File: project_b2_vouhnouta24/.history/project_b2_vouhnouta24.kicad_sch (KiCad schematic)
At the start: 13 parts, among them J1 AVR-ISP-10, J2 Micro_SD_Card, U1 ATmega328-P-A, U2 ADP2108AUJ-3.3, U3 TXB0104D, Y1 16Mhz

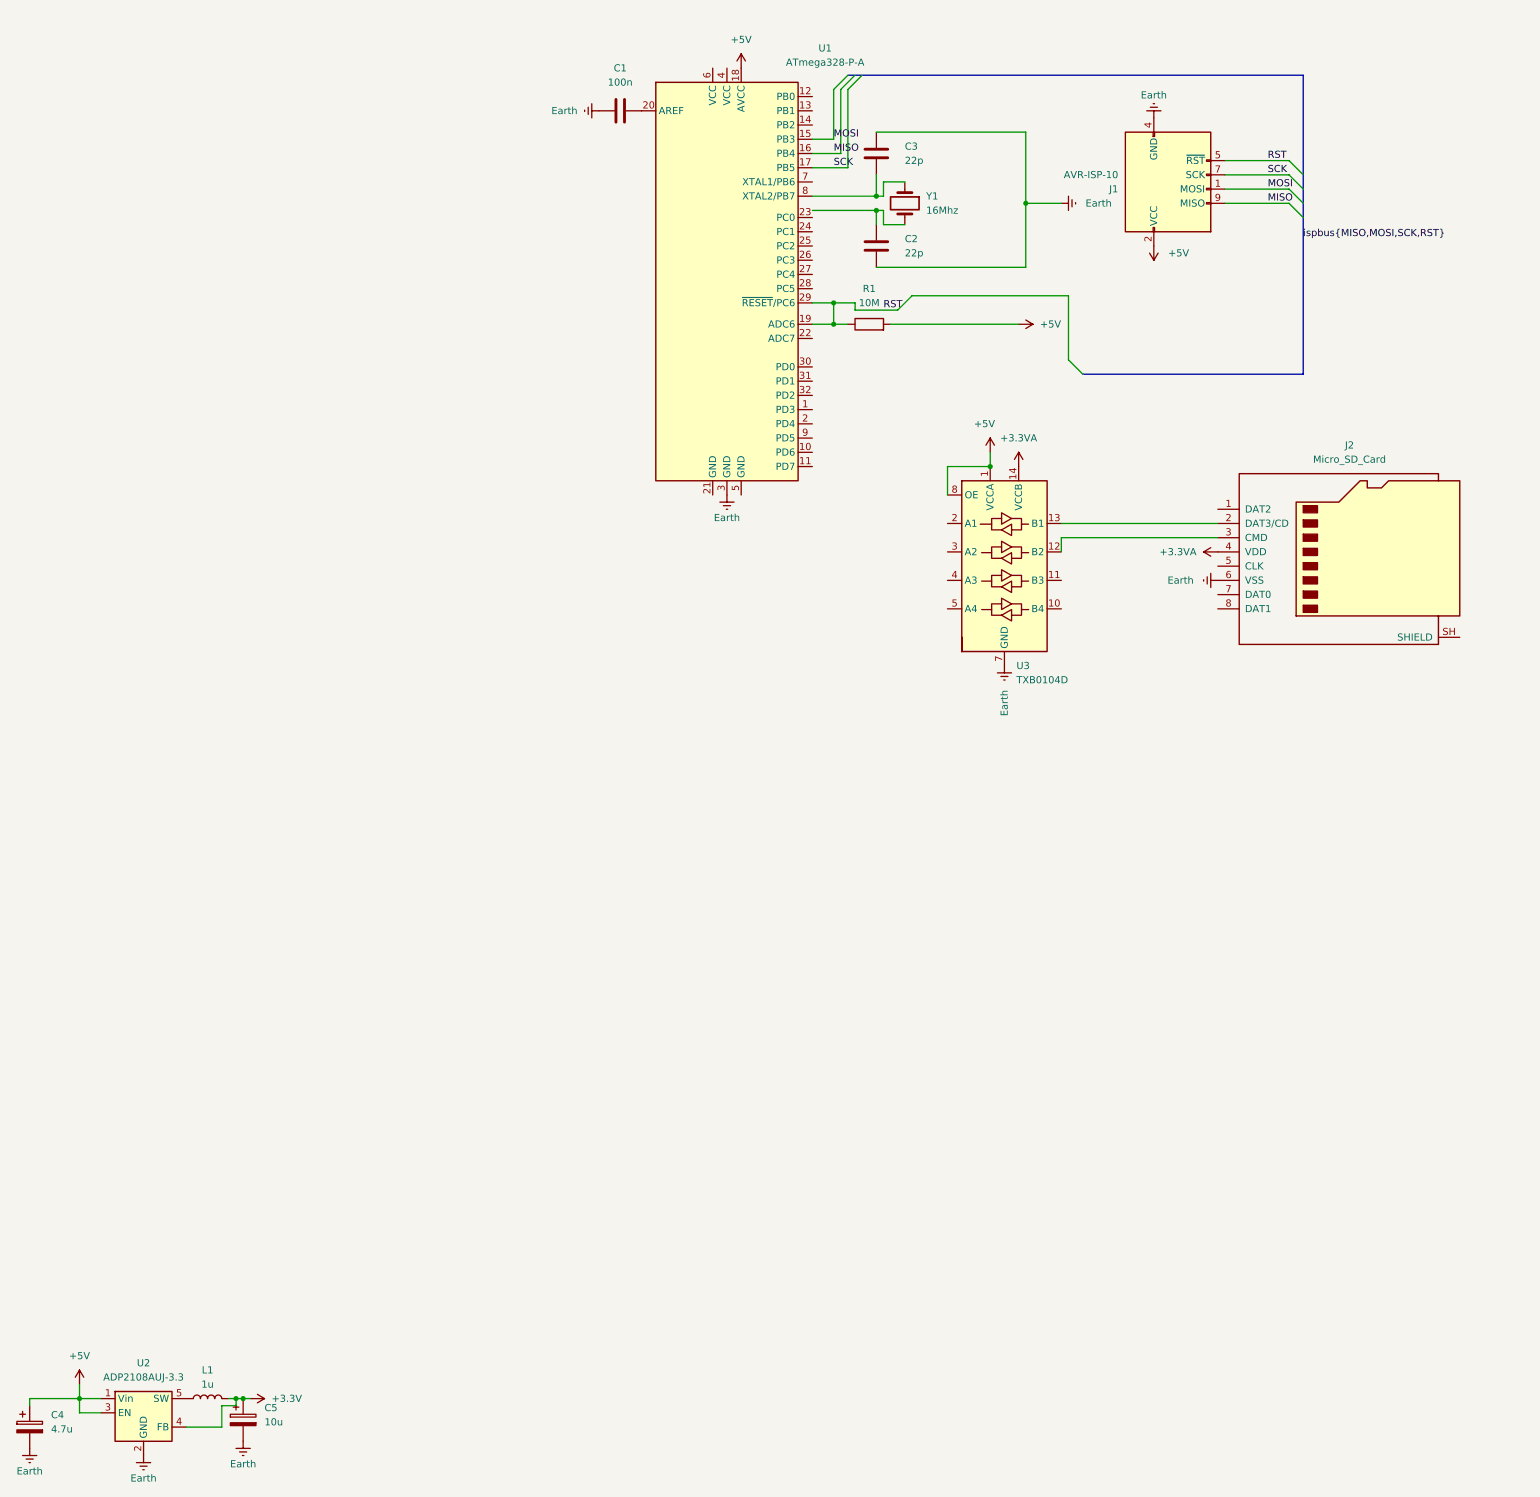
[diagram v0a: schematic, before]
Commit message: all the busses connected correctly finally
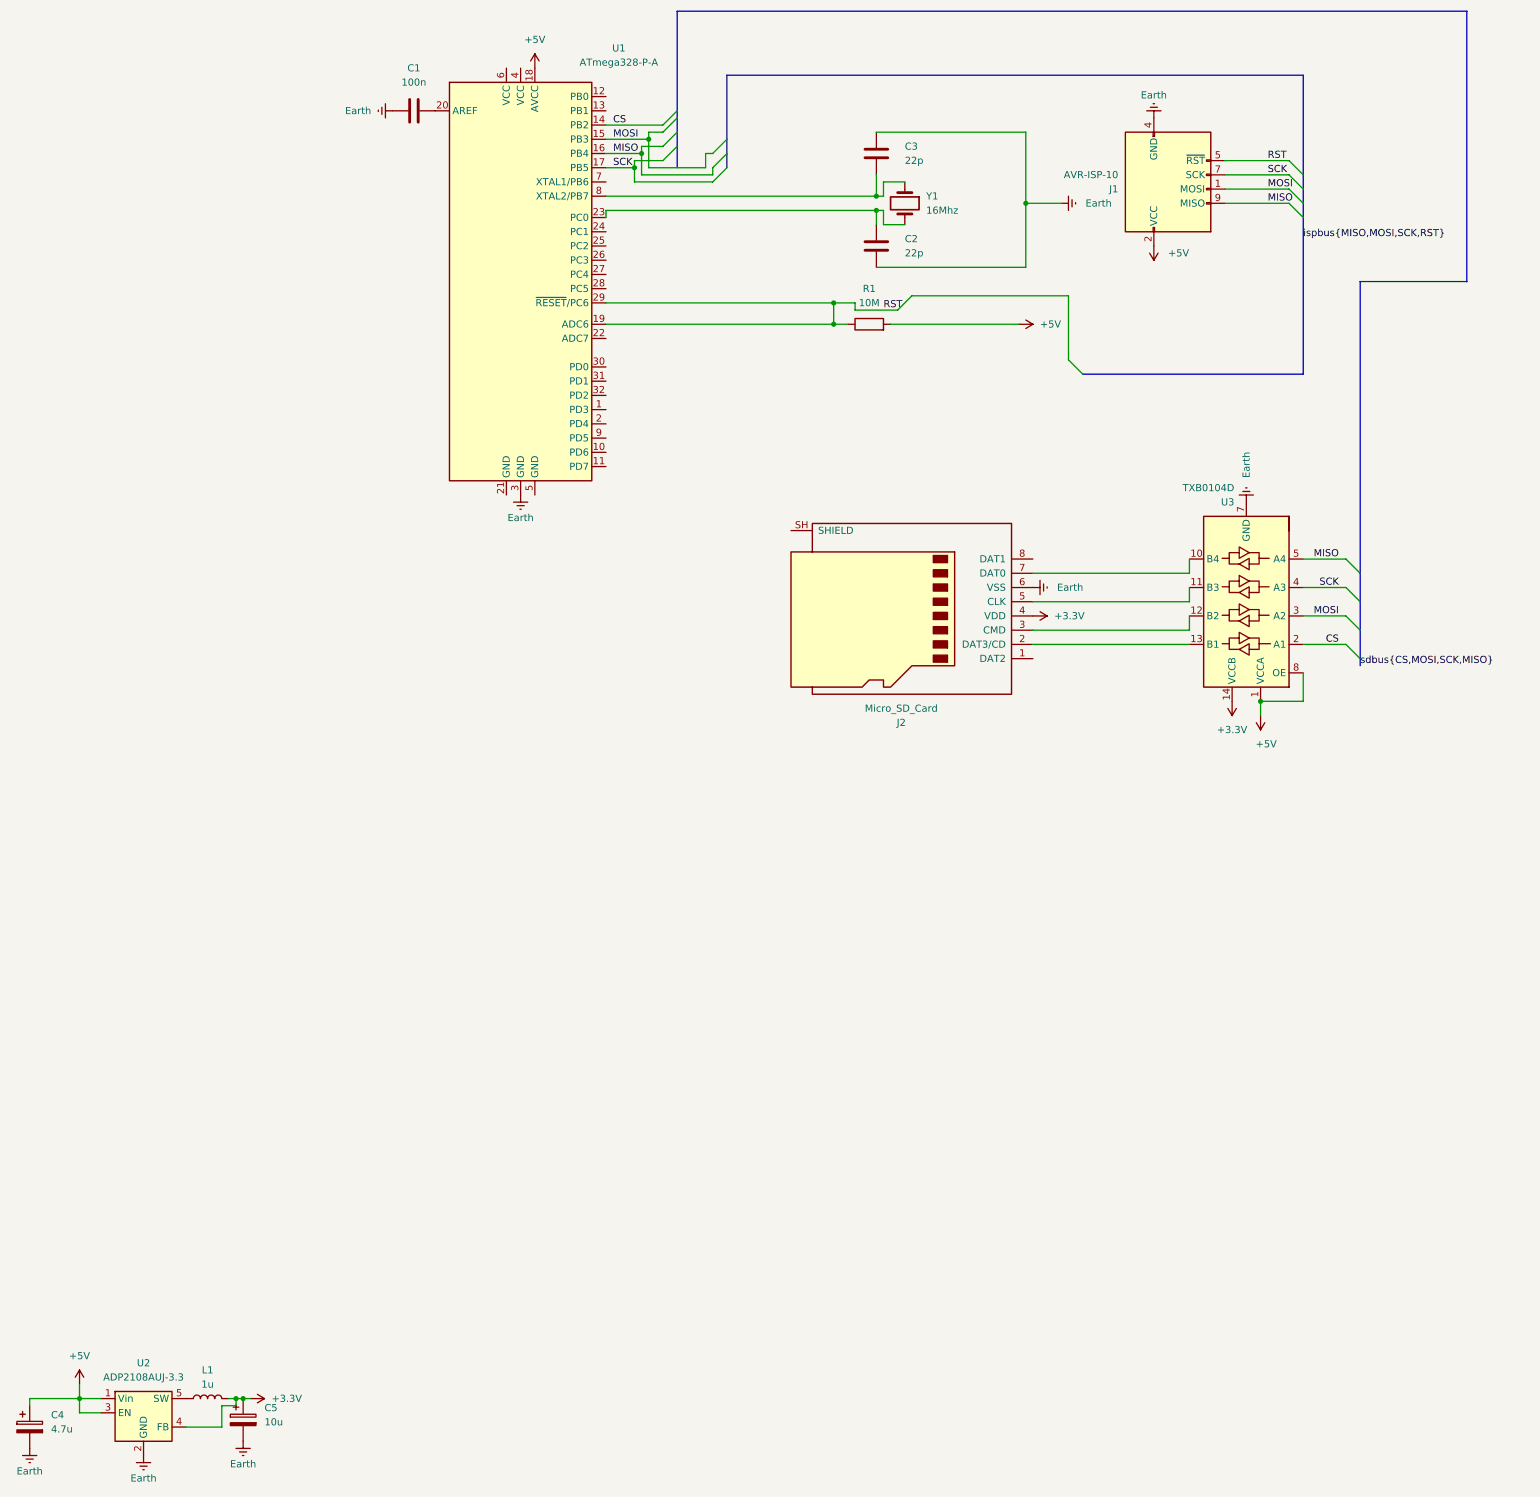
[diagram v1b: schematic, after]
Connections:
- net +3.3VA is gone; now on net +3.3V: J2.4 (VDD), U3.14 (VCCB)
- net MISO: now also U3.5 (A4)
- net MOSI: now also U3.3 (A2)
- net SCK: now also U3.4 (A3)
- net at C2.2, Y1.2: now also U1.23 (PC0)
- net at U3.10 (B4): now also J2.7 (DAT0)
- net at U3.11 (B3): now also J2.5 (CLK)
- net CS: now reaches U3.2 (A1)
- net CS: now also U1.14 (PB2)
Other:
- moved on the sheet: C1, J2, U1, U3
